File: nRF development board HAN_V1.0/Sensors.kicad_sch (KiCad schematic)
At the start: 7 parts, among them SW1 SW_Push, SW2 RotaryEncoder_Switch, U4 BME280, U5 BNO055

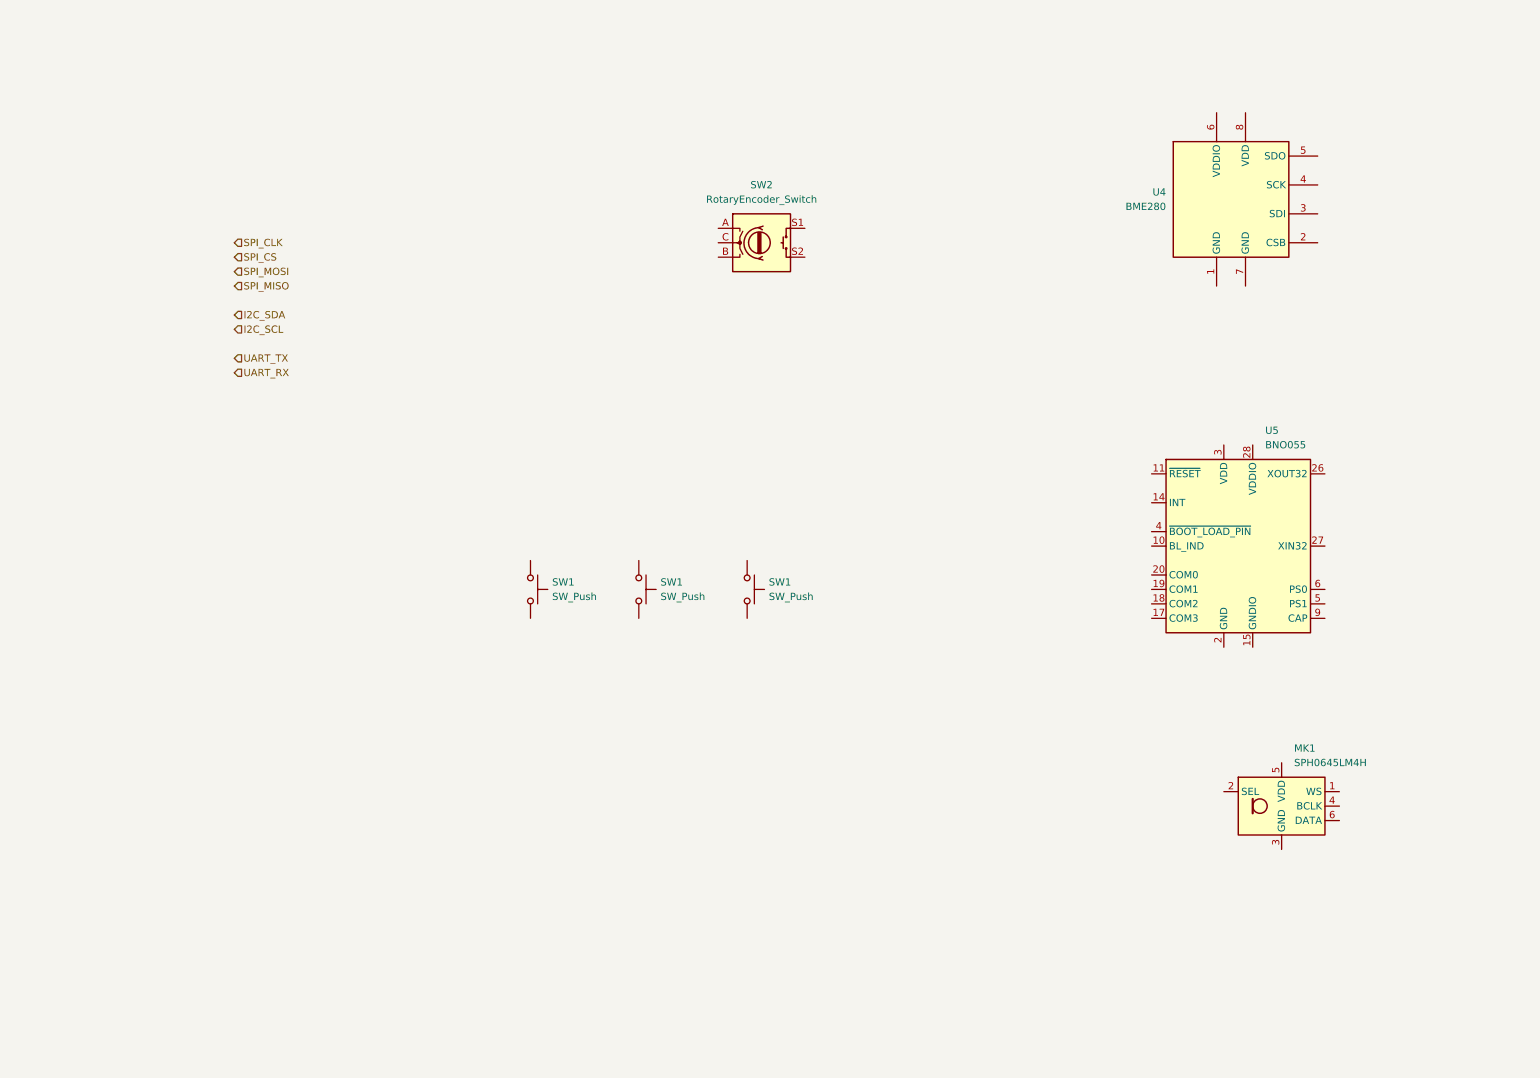
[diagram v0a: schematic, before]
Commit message: Updated schematic
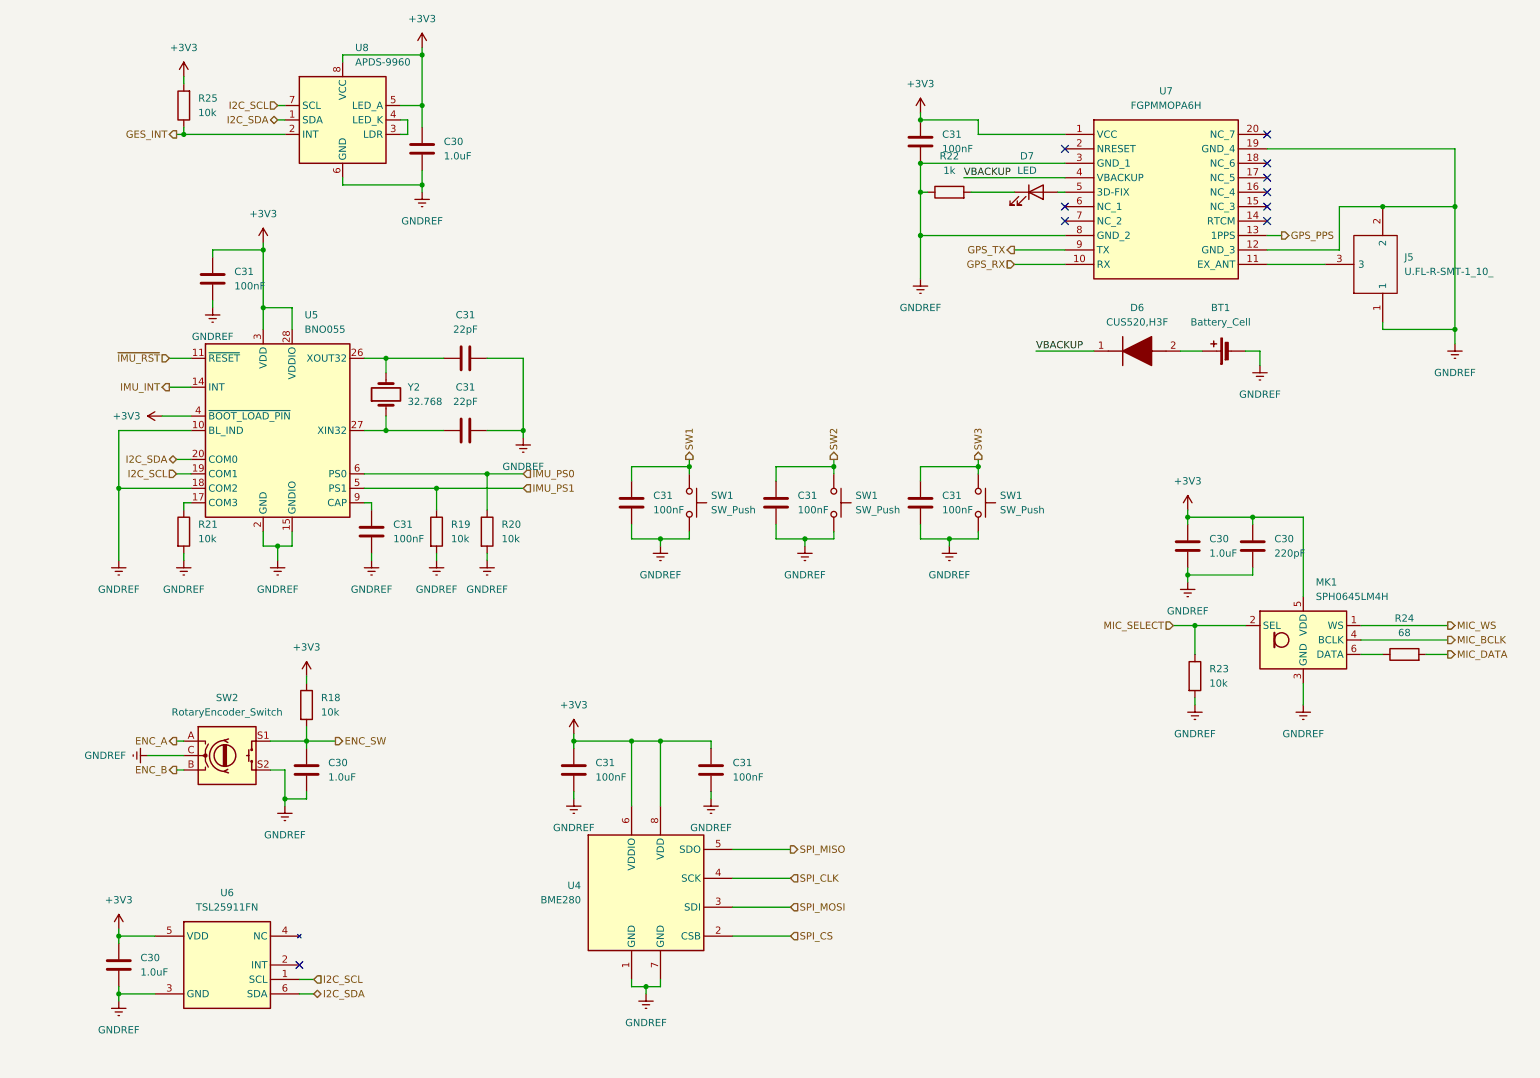
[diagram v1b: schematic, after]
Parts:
- added BT1: Battery_Cell, symbol Device:Battery_Cell
- added C30: 220pF, Capacitor_SMD:C_0603_1608Metric_Pad1.08x0.95mm_HandSolder, symbol Device:C
- added C30 (x4): 1.0uF, Capacitor_SMD:C_0603_1608Metric_Pad1.08x0.95mm_HandSolder, symbol Device:C
- added C31 (x2): 22pF, Capacitor_SMD:C_0603_1608Metric_Pad1.08x0.95mm_HandSolder, symbol Device:C
- added C31 (x8): 100nF, Capacitor_SMD:C_0603_1608Metric_Pad1.08x0.95mm_HandSolder, symbol Device:C
- added D6: CUS520,H3F, SOD2513X115N, symbol SamacSys_Parts:CUS520,H3F
- added D7: LED, symbol Device:LED
- added J5: U.FL-R-SMT-1_10_, U.FL-R-SMT-1(10), symbol SamacSys_Parts:U.FL-R-SMT-1_10_
- added R18, R19, R20, R21, R23, R25: 10k, symbol Device:R
- added R22: 1k, symbol Device:R
- added R24: 68, symbol Device:R
- added U6: TSL25911FN, TSL25911FN, symbol SamacSys_Parts:TSL25911FN
- added U7: FGPMMOPA6H, FGPMMOPA6H, symbol SamacSys_Parts:FGPMMOPA6H
- added U8: APDS-9960, Sensor:Avago_APDS-9960, symbol Sensor:APDS-9960
- added Y2: 32.768, symbol Device:Crystal
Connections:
- net I2C_SCL: now also U5.19 (COM1), U6.1 (SCL), U8.7 (SCL)
- net I2C_SDA: now also U5.20 (COM0), U6.6 (SDA), U8.1 (SDA)
- net SPI_CLK: now also U4.4 (SCK)
- net SPI_CS: now also U4.2 (CSB)
- net SPI_MISO: now also U4.5 (SDO)
- net SPI_MOSI: now also U4.3 (SDI)
- net SW1: now reaches SW1.1
- net SW1: now also C31.1
- net GNDREF: now reaches SW1.2
- net GNDREF: now also MK1.3 (GND), SW1.2, SW1.2, SW2.C, SW2.S2, U4.1 (GND), U4.7 (GND), U5.10 (BL_IND), U5.15 (GNDIO), U5.16 (GNDIO), U5.18 (COM2), U5.2 (GND), U5.25 (GNDIO), BT1.2 (-), C30.2, C30.2, C30.2, C30.2, C30.2, C31.2, C31.2, C31.2, C31.2, C31.2, C31.2, C31.2, C31.2, C31.2, C31.2, J5.1, J5.2, R19.2, R20.2, R21.2, R22.1, R23.2, U6.3 (GND), U7.12 (GND_3), U7.19 (GND_4), U7.3 (GND_1), U7.8 (GND_2), U8.6 (GND)
- net SW2: now reaches SW1.1
- net SW2: now also C31.1
- net ~{IMU_RST}: now reaches U5.11 (~{RESET})
- net IMU_INT: now reaches U5.14 (INT)
- net at U5.17 (COM3): now also R21.1
- net at U5.26 (XOUT32): now also C31.1, Y2.2
- net at U5.27 (XIN32): now also C31.1, Y2.1
- net +3V3: now reaches U5.28 (VDDIO)
- net +3V3: now also MK1.5 (VDD), U4.6 (VDDIO), U4.8 (VDD), U5.3 (VDD), U5.4 (~{BOOT_LOAD_PIN}), C30.1, C30.1, C30.1, C30.1, C31.1, C31.1, C31.1, C31.1, R18.1, R25.2, U6.5 (VDD), U7.1 (VCC), U8.5 (LED_A), U8.8 (VCC)
- net IMU_PS1: now reaches U5.5 (PS1)
- net IMU_PS1: now also R19.1
- net IMU_PS0: now reaches U5.6 (PS0)
- net IMU_PS0: now also R20.1
- net at U5.9 (CAP): now also C31.1
- net SW3: now reaches SW1.1
- net SW3: now also C31.1
- net ENC_A: now reaches SW2.A
- net ENC_B: now reaches SW2.B
- net ENC_SW: now reaches SW2.S1
- net ENC_SW: now also C30.1, R18.2
- net MIC_WS: now reaches MK1.1 (WS)
- net MIC_SELECT: now reaches MK1.2 (SEL)
- net MIC_SELECT: now also R23.1
- net MIC_BCLK: now reaches MK1.4 (BCLK)
- net at MK1.6 (DATA): now also R24.1
- new net: BT1.1 (+), D6.2 (A)
- new net: J5.3, U7.11 (EX_ANT)
- new net: D7.2 (A), U7.5 (3D-FIX)
- new net: D7.1 (K), R22.2
- new net: U8.3 (LDR), U8.4 (LED_K)
- new net GES_INT: R25.1, U8.2 (INT)
- new net GPS_PPS: U7.13 (1PPS)
- new net GPS_RX: U7.10 (RX)
- new net GPS_TX: U7.9 (TX)
- new net MIC_DATA: R24.2
- new net VBACKUP: D6.1 (K), U7.4 (VBACKUP)
- no-connect marks 0 -> 10
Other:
- moved on the sheet: MK1, SW1, SW2, U4, U5

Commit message: QOL update
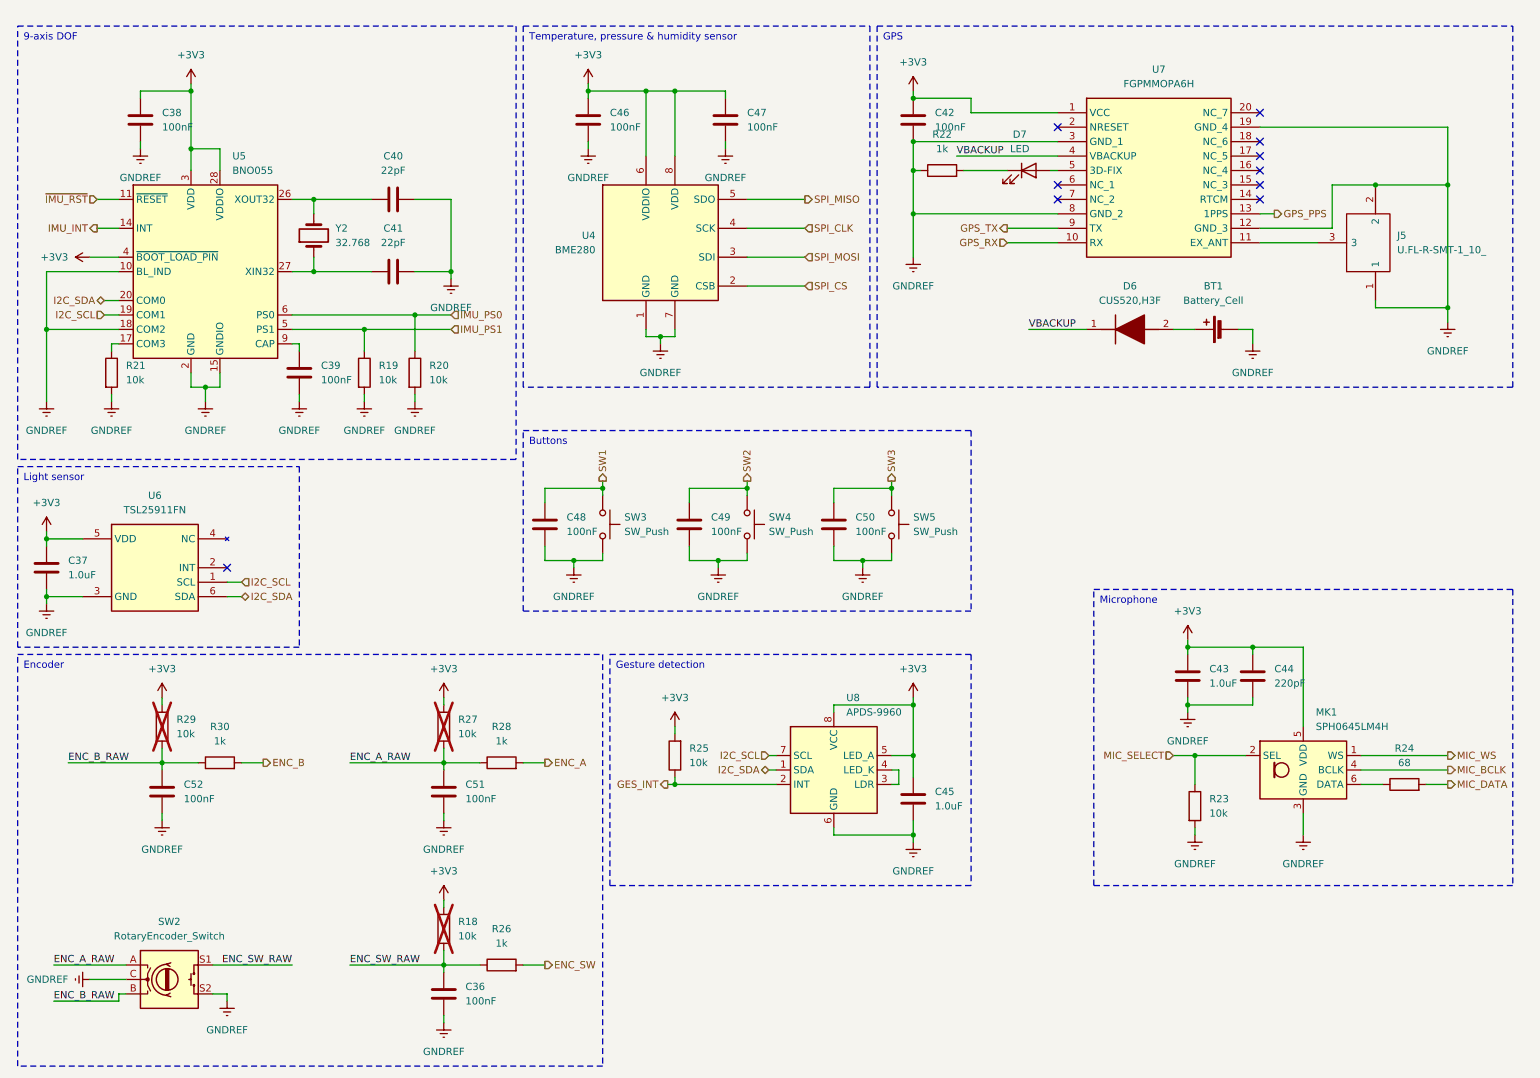
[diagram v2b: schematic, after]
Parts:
- added C51, C52: 100nF, Capacitor_SMD:C_0603_1608Metric_Pad1.08x0.95mm_HandSolder, symbol Device:C
- added R26, R28, R30: 1k, symbol Device:R
- added R27, R29: 10k, symbol Device:R
- C36: renamed from C30; value 1.0uF -> 100nF
- R18: now not fitted; now left out of the parts list
- renumbered C30 to C37, C31 to C38, C31 to C39, C31 to C40, C31 to C41, C31 to C42, C30 to C43, C30 to C44, C30 to C45, C31 to C46, C31 to C47, C31 to C48, C31 to C49, C31 to C50, SW1 to SW3, SW1 to SW4, SW1 to SW5
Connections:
- net +3V3: now also R27.1, R29.1
- net ENC_A: now also R28.2; no longer SW2.A
- net ENC_B: now also R30.2; no longer SW2.B
- net ENC_SW: now also R26.2; no longer C36.1, R18.2, SW2.S1
- net GNDREF: now also C51.2, C52.2
- new net ENC_A_RAW: C51.1, R27.2, R28.1, SW2.A
- new net ENC_B_RAW: C52.1, R29.2, R30.1, SW2.B
- new net ENC_SW_RAW: C36.1, R18.2, R26.1, SW2.S1
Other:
- moved on the sheet: BT1, C36, C37, C38, C39, C40, C41, C42, C43, C44, C45, C46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
